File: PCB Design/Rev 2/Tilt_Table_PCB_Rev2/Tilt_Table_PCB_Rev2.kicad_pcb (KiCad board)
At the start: 4 copper layers, 47 x 60 mm, 70 parts, among them J1 2171750001, J10 X_SERVO_HDR, J11 Touch_Panel_HDR, J2 7x1 RECP, J3 PD_Output, J4 BUCK_EN, J5 MCU_Header, J6 BOOT_HDR, J7 SWD, J8 USB_B_Micro, J9 Y_SERVO_HDR, Q1 DMP3098LSD-13, Q2 2N7002, SW1 RST_BTN, U1 CYPD3177-24LQ, U2 TPS54531DDA, U3 TLV75533PDBV, U4 STM32C071FBPx

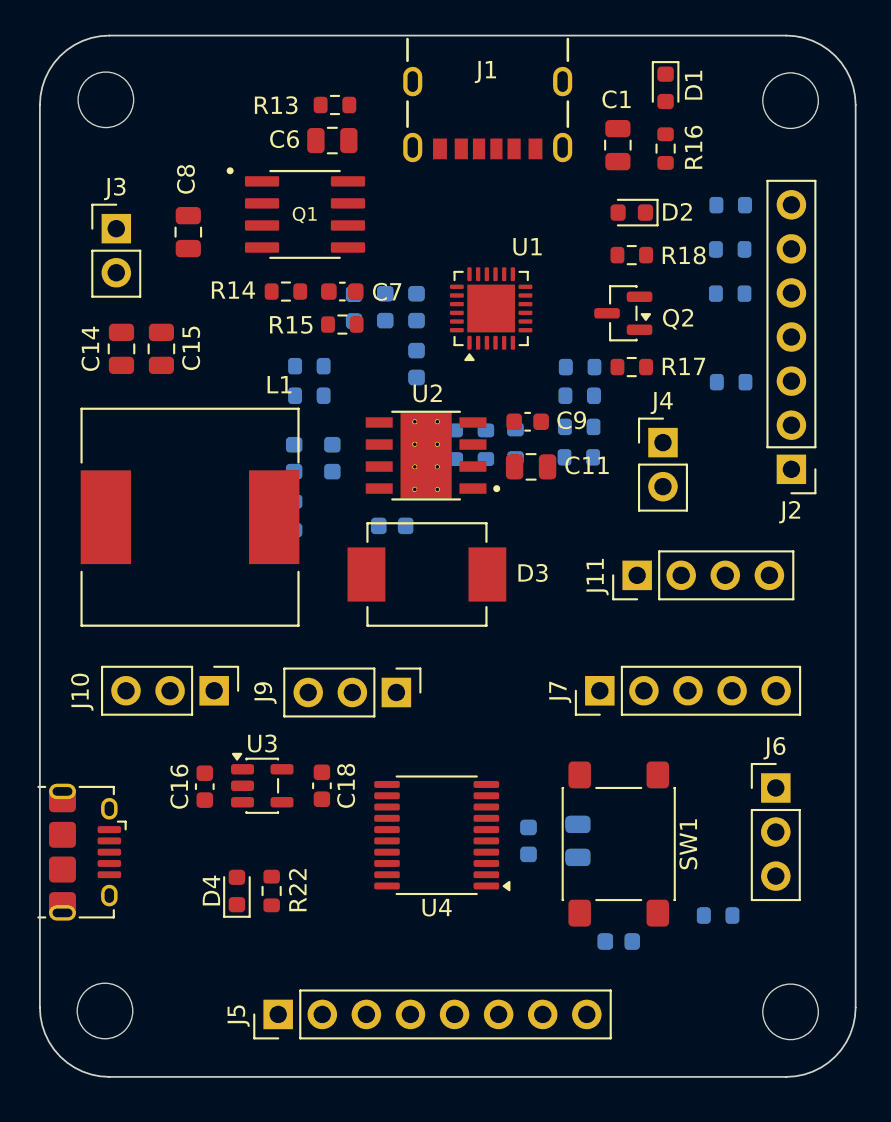
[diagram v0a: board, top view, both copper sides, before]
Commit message: PCB Rev 2 Update
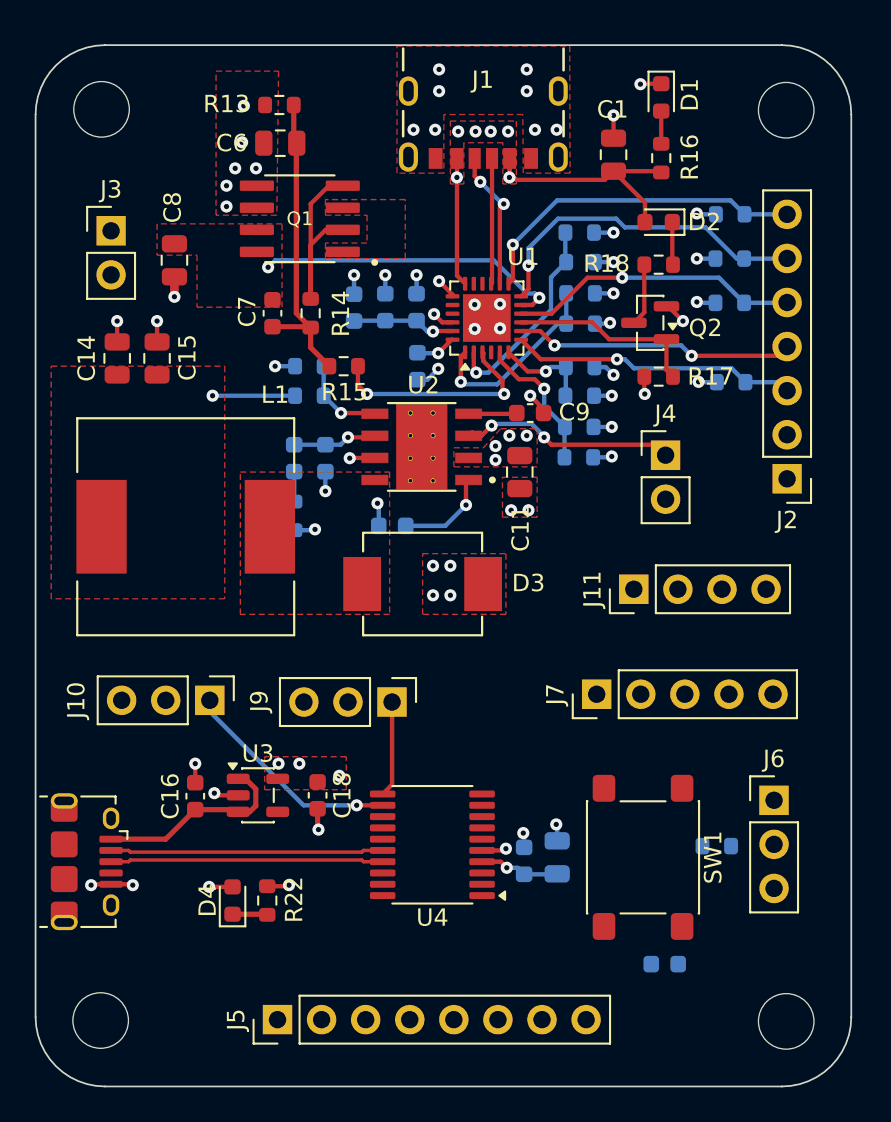
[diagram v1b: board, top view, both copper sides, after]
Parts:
- moved R1 12.7 mm to (151.4, 35.8), turned to 180 degrees
- moved R2 11.9 mm to (151.5, 37.5), turned to 0 degrees
- moved R6 11.4 mm to (151.5, 41.0), turned to 0 degrees
- moved R5 11.3 mm to (151.5, 39.3), turned to 180 degrees
- moved C7 4.21 mm to (133.8, 40.5), turned to -90 degrees
- moved R23 4.00 mm to (159.3, 71.2)
- moved R13 3.20 mm to (134.2, 28.4), turned to 0 degrees
- moved C6 3.00 mm to (134.2, 30.6), turned to 0 degrees
- moved C17 2.95 mm to (156.3, 78.0)
- moved R15 2.40 mm to (137.8, 43.5)
- moved R14 1.90 mm to (135.9, 40.5), turned to -90 degrees
- moved C8 1.81 mm to (128.1, 37.4)
- moved D2 1.64 mm to (156.0, 35.2)
- moved R17 1.64 mm to (156.0, 44.1)
- moved R18 1.64 mm to (156.0, 37.6), turned to 180 degrees
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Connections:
- net Net-(J8-D+) renamed /MCU/USB_D+
- net Net-(J8-D-) renamed /MCU/USB_D-
- J5 pad 3: /MCU/UART_TX -> /MCU/PA7
- J5 pad 4: /MCU/UART_RX -> /MCU/PA8
- J5 pad 5: /MCU/PA7 -> /MCU/PB3/4/5/6
- J5 pad 6: /MCU/PA8 -> /MCU/PC15
- J5 pad 7: /MCU/PC15 -> /MCU/UART_TX
- J5 pad 8: /MCU/PB3/4/5/6 -> /MCU/UART_RX
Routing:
- net GND: track 0.00 -> 37.4 mm, vias 0 -> 49
- net VBUS_IN: track 0.00 -> 23.0 mm, vias 0 -> 12
- net /Power/HPI_SCL: track 0.00 -> 19.5 mm, vias 0 -> 1
- net /Power/HPI_SDA: track 0.00 -> 19.5 mm, vias 0 -> 1
- net /Power/VBUS_FET_EN_R: track 0.00 -> 18.1 mm
- net VBUS_OUT: track 0.00 -> 18.1 mm, vias 0 -> 6
- net /Power/FLIP: track 0.00 -> 16.8 mm, vias 0 -> 1
- net /Power/SWD_IO_INT: track 0.00 -> 16.5 mm, vias 0 -> 1
- net /Power/SWD_CLK: track 0.00 -> 16.1 mm, vias 0 -> 2
- net /MCU/USB_D-: track 0.00 -> 15.7 mm
- net /MCU/USB_D+: track 0.00 -> 15.7 mm
- net PDC_3.3V: track 0.00 -> 14.8 mm, vias 0 -> 9
- net /Power/VBUS_FET_G: track 0.00 -> 13.1 mm
- net /MCU/SERVO_X: track 0.00 -> 12.8 mm, vias 0 -> 1
- net Net-(J4-Pin_1): track 0.00 -> 12.7 mm, vias 0 -> 2
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- added copper zone on F.Cu, net +3.3V
- added copper zone on In2.Cu, net +3.3V
- added copper zone on F.Cu, net +6V
- added copper zone on In2.Cu, net +6V
- added copper zone on F.Cu, net /Power Conversion/PH
- added copper zone on In2.Cu, net /Power Conversion/PH
- added copper zone on F.Cu, net /Power/FET_SRC
- added copper zone on F.Cu, net GND
- added copper zone on In1.Cu, net GND
- added copper zone on In2.Cu, net PDC_3.3V
- added copper zone on F.Cu, net VBUS_IN
- added copper zone on In2.Cu, net VBUS_IN
- added copper zone on F.Cu, net VBUS_OUT
- added copper zone on In2.Cu, net VBUS_OUT
